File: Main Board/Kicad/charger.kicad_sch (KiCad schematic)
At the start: 12 parts, among them U8 LT3652IMSE

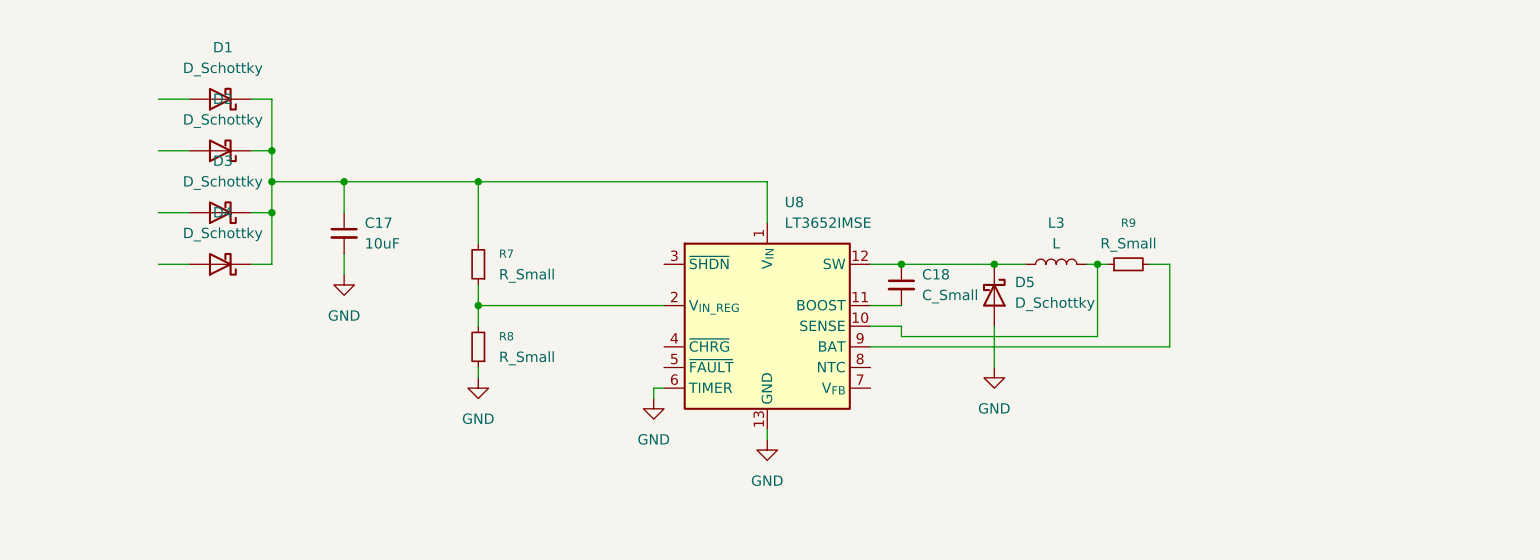
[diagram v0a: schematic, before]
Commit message: Atualização do circuito/pcb
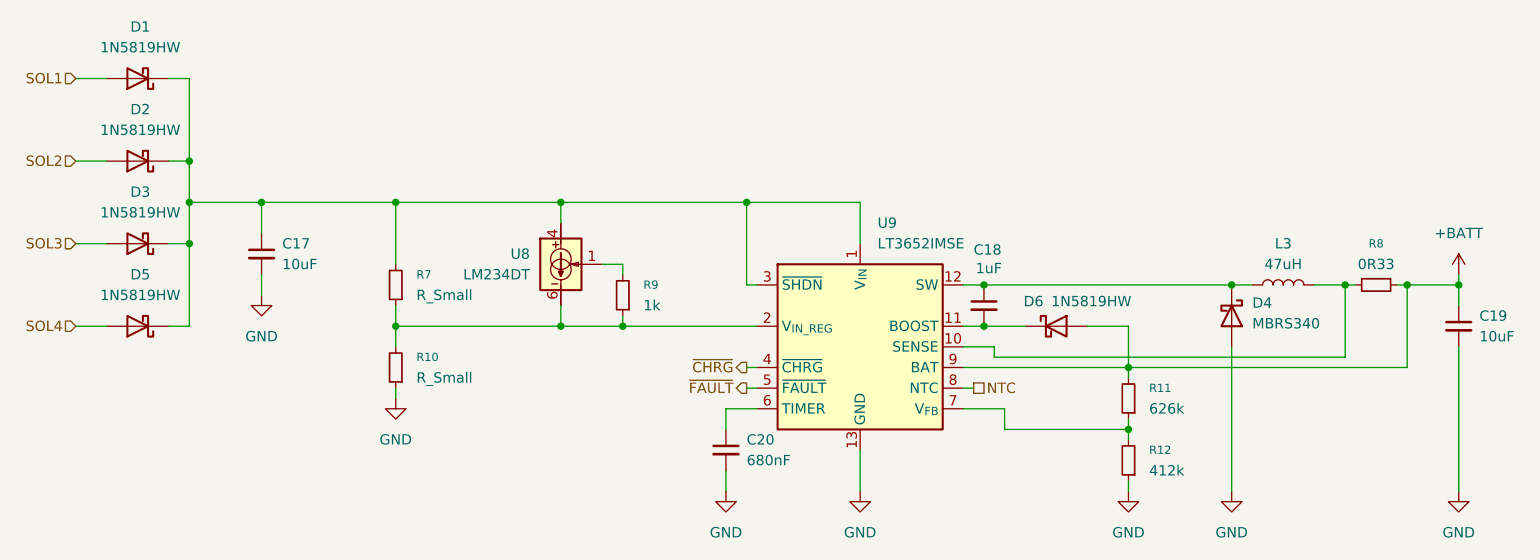
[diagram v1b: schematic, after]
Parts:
- removed D5: D_Schottky, symbol Device:D_Schottky
- added C19: 10uF, Capacitor_SMD:C_1206_3216Metric_Pad1.33x1.80mm_HandSolder, symbol Device:C_Small
- added C20: 680nF, Capacitor_SMD:C_0402_1005Metric_Pad0.74x0.62mm_HandSolder, symbol Device:C_Small
- added D4: MBRS340, Diode_SMD:D_SMC, symbol Diode:MBRS340
- added D6: 1N5819HW, Diode_SMD:D_SOD-123, symbol Device:D_Schottky
- added R11: 626k, Resistor_SMD:R_0402_1005Metric_Pad0.72x0.64mm_HandSolder, symbol Device:R_Small
- added R12: 412k, Resistor_SMD:R_0402_1005Metric_Pad0.72x0.64mm_HandSolder, symbol Device:R_Small
- added R9: 1k, Resistor_SMD:R_0402_1005Metric_Pad0.72x0.64mm_HandSolder, symbol Device:R_Small
- added U8: LM234DT, Package_SO:SOIC-8_3.9x4.9mm_P1.27mm, symbol Reference_Current:LM234Z-3
- C17: footprint (none) -> Capacitor_SMD:C_1206_3216Metric_Pad1.33x1.80mm_HandSolder
- C18: value C_Small -> 1uF; footprint (none) -> Capacitor_SMD:C_0402_1005Metric_Pad0.74x0.62mm_HandSolder
- D1, D2, D3: value D_Schottky -> 1N5819HW; footprint (none) -> Diode_SMD:D_SOD-123
- D5: renamed from D4; value D_Schottky -> 1N5819HW; footprint (none) -> Diode_SMD:D_SOD-123
- L3: value L -> 47uH; footprint (none) -> Inductor_SMD:L_TDK_SLF7032
- R10: renamed from R8; footprint (none) -> Resistor_SMD:R_0402_1005Metric_Pad0.72x0.64mm_HandSolder
- R7: footprint (none) -> Resistor_SMD:R_0402_1005Metric_Pad0.72x0.64mm_HandSolder
- R8: renamed from R9; value R_Small -> 0R33; footprint (none) -> Resistor_SMD:R_1210_3225Metric_Pad1.30x2.65mm_HandSolder
- renumbered U8 to U9
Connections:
- net GND: now also C19.2, C20.2, D4.2 (A), R12.1; no longer U9.6 (TIMER)
- net at C17.1, D1.1 (K), D2.1 (K)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: now also U9.3 (~{SHDN}), U8.4
- net SOL4: now reaches D5.2 (A)
- net at R10.2, R7.1, U9.2 (V_{IN_REG}): now also R9.1, U8.6
- net +BATT: now reaches R8.2, U9.9 (BAT)
- net +BATT: now also C19.1, D6.2 (A), R11.2
- net SOL3: now reaches D3.2 (A)
- net at C18.2, U9.11 (BOOST): now also D6.1 (K)
- net at C18.1, L3.1, U9.12 (SW): now also D4.1 (K)
- net ~{CHRG}: now reaches U9.4 (~{CHRG})
- net ~{FAULT}: now reaches U9.5 (~{FAULT})
- net at U9.7 (V_{FB}): now also R11.1, R12.2
- net NTC: now reaches U9.8 (NTC)
- net SOL1: now reaches D1.2 (A)
- net SOL2: now reaches D2.2 (A)
- new net: R9.2, U8.1
- new net: C20.1, U9.6 (TIMER)
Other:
- moved on the sheet: C17, C18, D1, D2, D3, D5, L3, R10, R7, R8, U9
